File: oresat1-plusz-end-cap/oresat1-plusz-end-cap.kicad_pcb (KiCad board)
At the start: 4 copper layers, 105.6 x 105.6 mm, 55 parts, among them J1 M55-7011242R, J2 U.FL-R-SMA, U1 RM3100, U2 RM3100

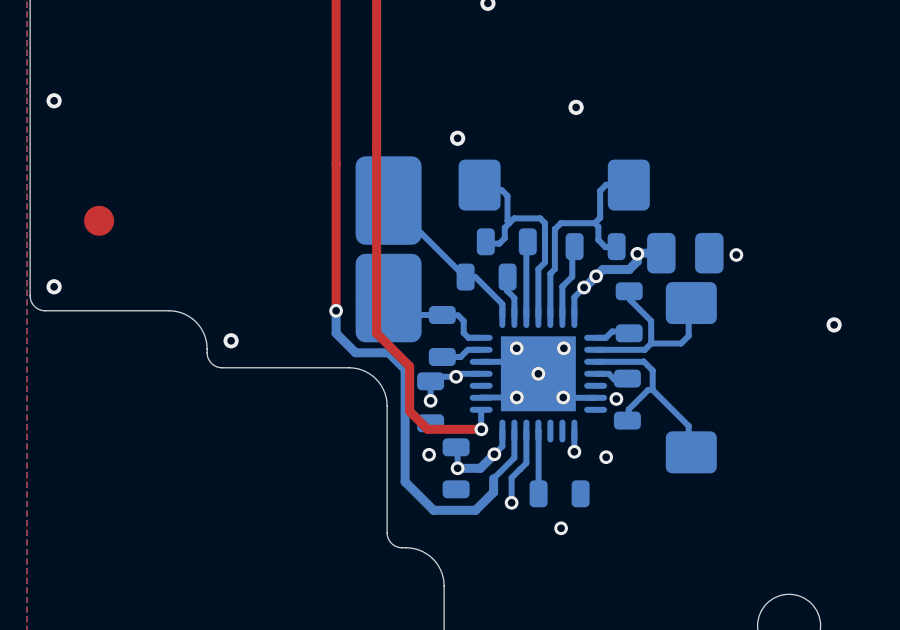
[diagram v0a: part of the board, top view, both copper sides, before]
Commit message: routine push
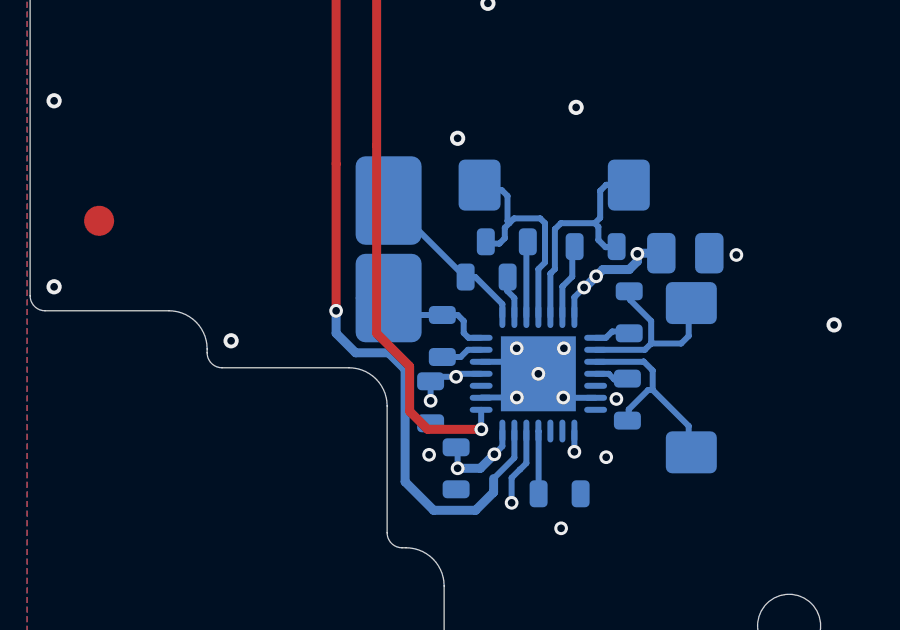
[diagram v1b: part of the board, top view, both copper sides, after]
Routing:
- net Net-(U1-ZINP): track 4.15 -> 4.67 mm
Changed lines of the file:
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@@
+	)
+	(segment
+		(start 110.745 146.89)
+		(end 111.9225 146.89)
+		(width 0.2)
+		(layer "B.Cu")
+		(net "GND")
 	)
 	(segment
@@
 	)
 	(segment
-		(start 110.745 146.89)
-		(end 111.9225 146.89)
-		(width 0.2)
-		(layer "B.Cu")
-		(net "GND")
-	)
-	(segment
 		(start 114.55 146.9)
 		(end 113.4825 146.9)
@@
 	)
 	(segment
+		(start 110.3125 144.9)
+		(end 110.1525 144.74)
+		(width 0.2)
+		(layer "B.Cu")
+		(net "Net-(U1-ZINP)")
+	)
+	(segment
 		(start 109.44 144.14)
 		(end 108.215 144.14)
@@
 	)
 	(segment
+		(start 110.735 144.9)
+		(end 110.3125 144.9)
+		(width 0.2)
+		(layer "B.Cu")
+		(net "Net-(U1-ZINP)")
+	)
+	(segment
+		(start 109.9525 144.14)
+		(end 109.44 144.14)
+		(width 0.2)
+		(layer "B.Cu")
+		(net "Net-(U1-ZINP)")
+	)
+	(segment
 		(start 110.1525 144.34)
 		(end 109.9525 144.14)
@@
 	)
 	(segment
-		(start 110.3125 144.9)
-		(end 110.1525 144.74)
-		(width 0.2)
-		(layer "B.Cu")
-		(net "Net-(U1-ZINP)")
-	)
-	(segment
 		(start 108.215 144.14)
 		(end 107.65 143.575)
 		(width 0.2)
 		(layer "B.Cu")
-		(net "Net-(U1-ZINP)")
-	)
-	(segment
-		(start 110.735 144.9)
-		(end 110.3125 144.9)
-		(width 0.2)
-		(layer "B.Cu")
